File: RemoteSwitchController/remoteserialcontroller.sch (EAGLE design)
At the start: 37 parts, among them J1 ZX62R-AB-5P, J2 D-SUB9, Q2 MMSS8050-L, Q3 MMSS8050-L, SW1 SKRPACE010, SW2 SKRPACE010, U1 ADM3202ARUZ, U2 ESP-WROOM-32, U21 FT232RL

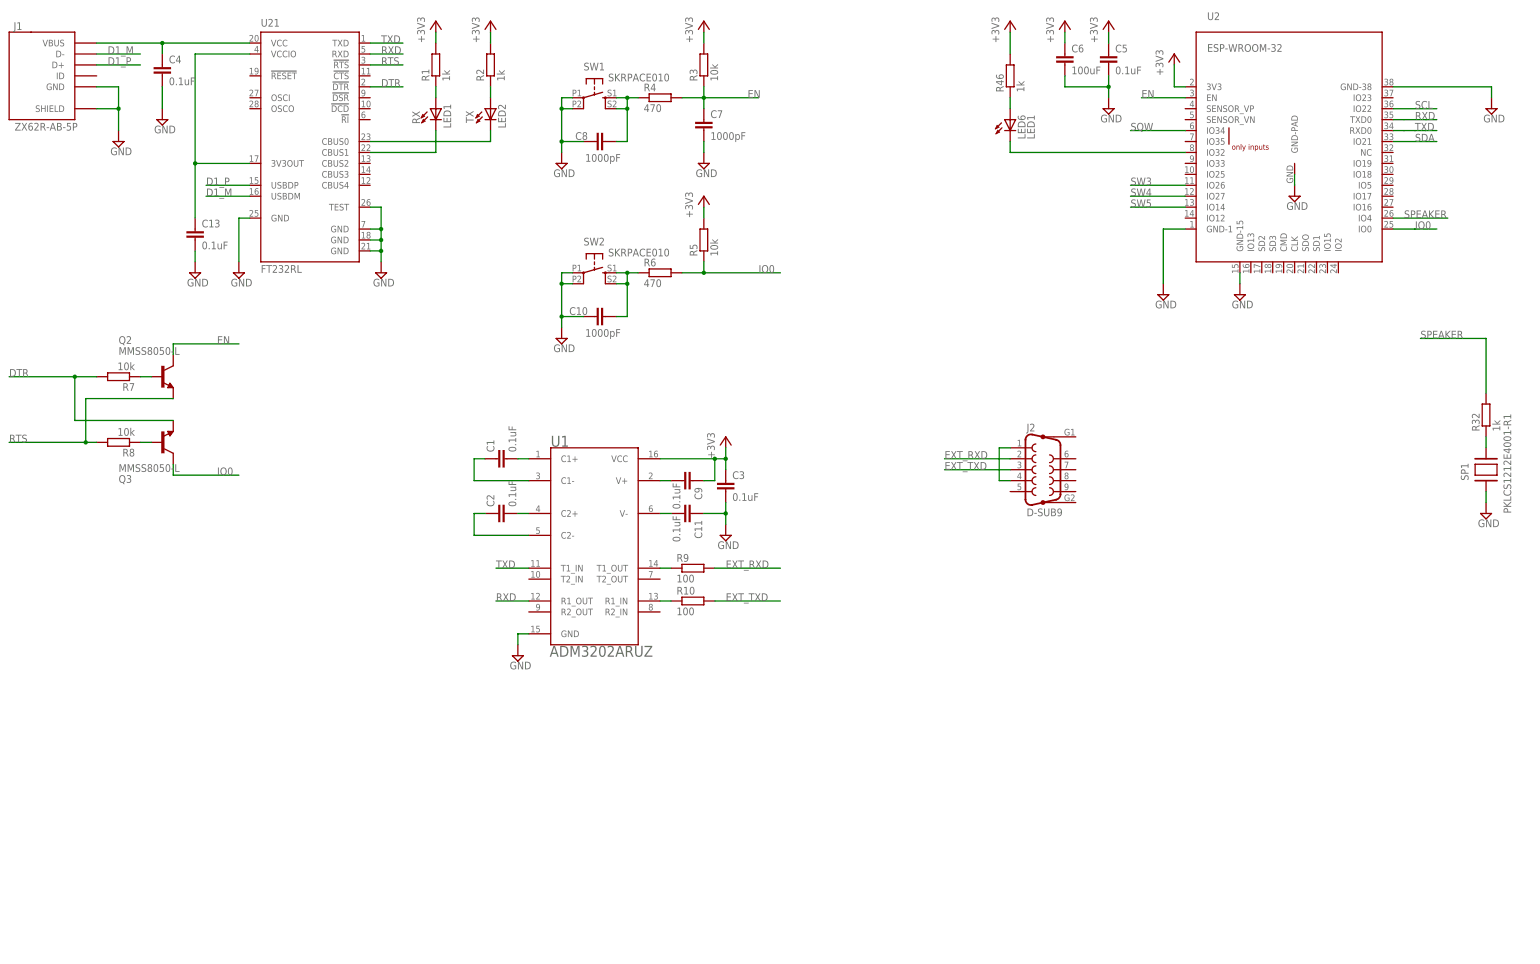
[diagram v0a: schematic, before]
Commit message: [add] temporrary
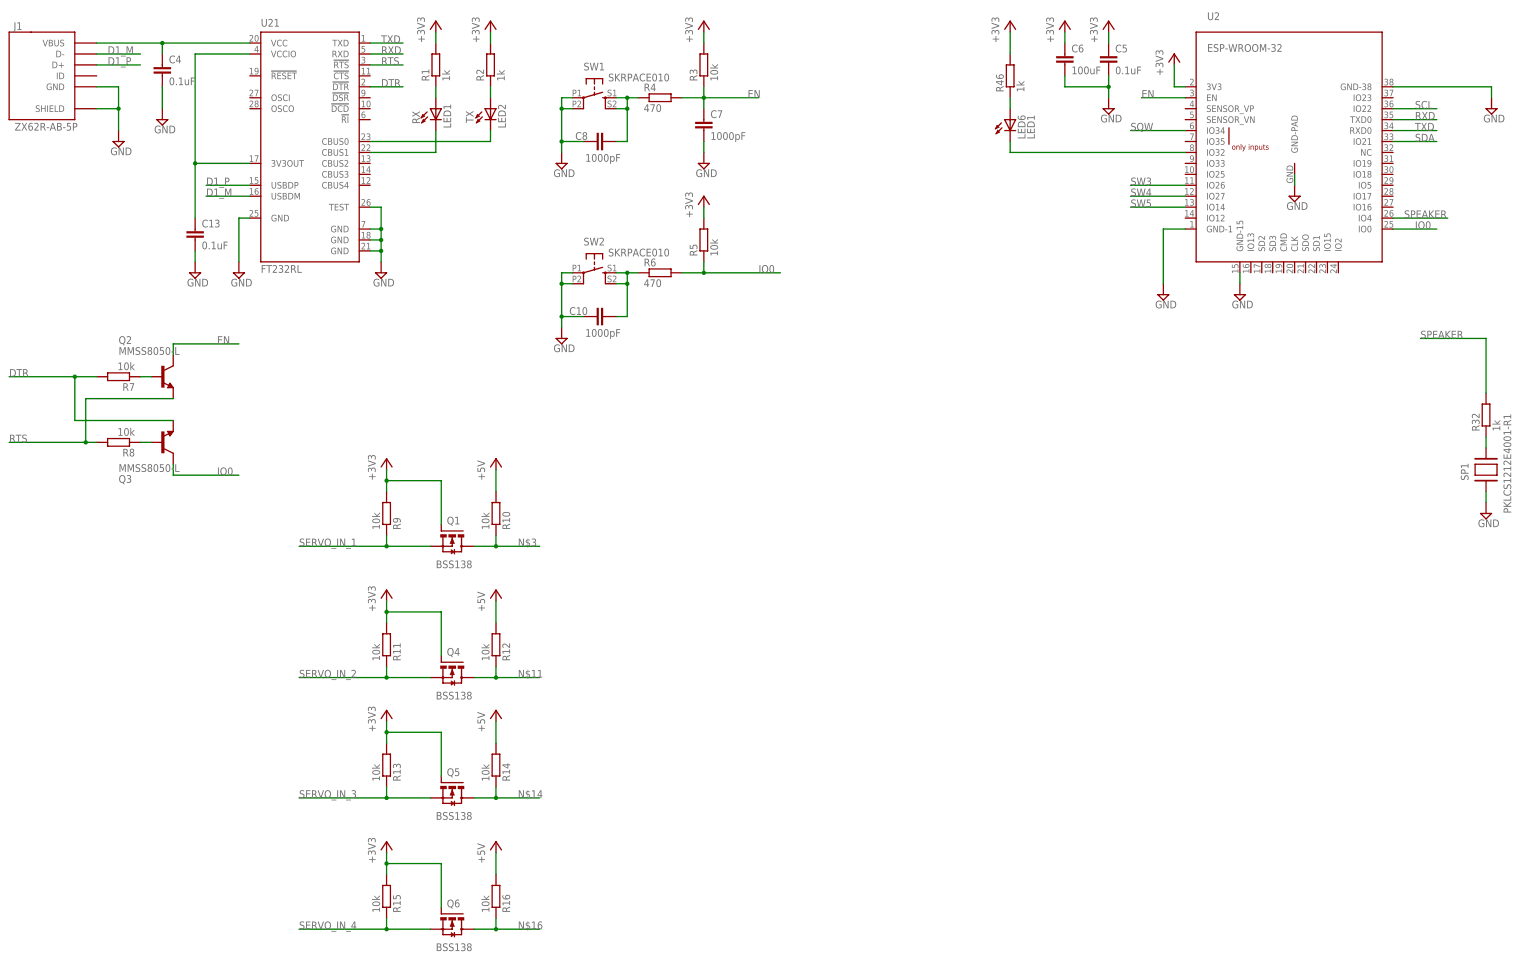
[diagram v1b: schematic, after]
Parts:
- removed C1, C11, C2, C3, C9: 0.1uF, taki-library:C-EUC0603
- removed J2: D-SUB9, taki-library:D-SUB9
- removed U1: ADM3202ARUZ, taki-library:ADM3202ARUZ
- added Q1, Q4, Q5, Q6: BSS138, taki-library:BSS138
- added R11, R12, R13, R14, R15, R16: 10k, taki-library:R-EU_R0603
- R10, R9: value 100 -> 10k
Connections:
- removed net EXT_RXD: J2.2, R9.2
- removed net EXT_TXD: J2.3, R10.2
- removed net N$1: J2.1, J2.4
- removed net N$13: C1.1, U1.C1-
- removed net N$15: C2.1, U1.C2-
- removed net N$17: C11.2, U1.V-
- removed net N$2: R9.1, U1.T1_OUT
- new net +5V: R10.2, R12.2, R14.2, R16.2
- new net SERVO_IN_1: Q1.S, R9.1
- new net SERVO_IN_2: Q4.S, R11.1
- new net SERVO_IN_3: Q5.S, R13.1
- new net SERVO_IN_4: Q6.S, R15.1
- net +3V3: now also Q1.G, Q4.G, Q5.G, Q6.G, R11.2, R13.2, R15.2, R9.2; no longer C3.1, C9.1, U1.VCC
- net GND: no longer C11.1, C3.2, U1.GND
- net N$11: now also Q4.D, R12.1; no longer C1.2, U1.C1+
- net N$14: now also Q5.D, R14.1; no longer C2.2, U1.C2+
- net N$16: now also Q6.D, R16.1; no longer C9.2, U1.V+
- net N$3: now also Q1.D; no longer U1.R1_IN
- net RXD: no longer U1.R1_OUT
- net TXD: no longer U1.T1_IN
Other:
- moved on the sheet: R10, R9

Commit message: [add]add all
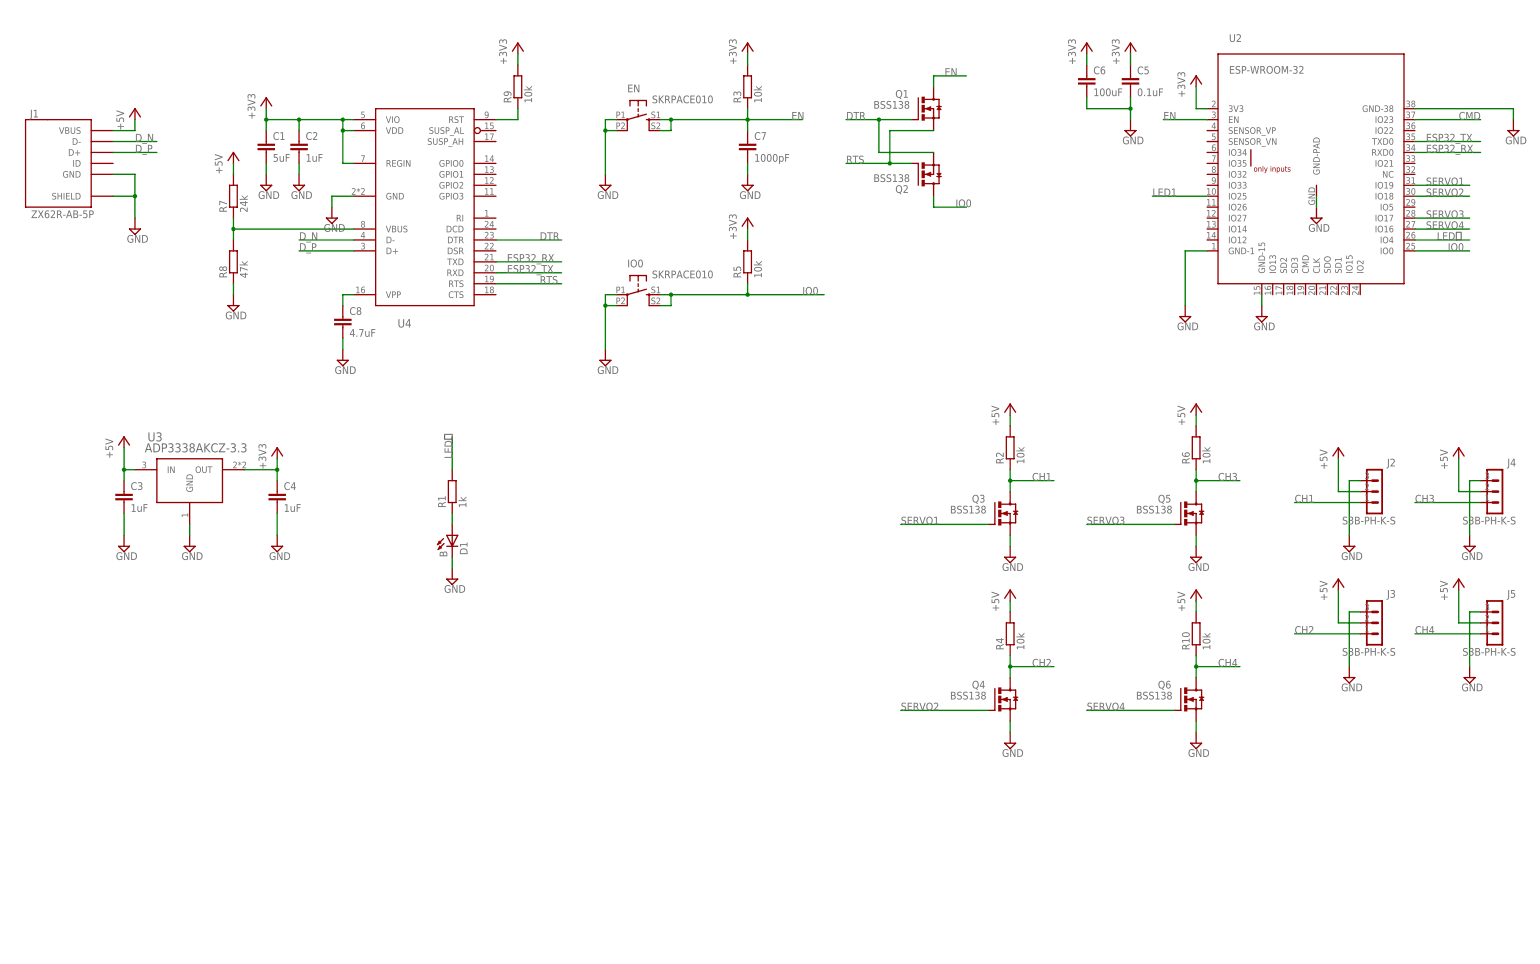
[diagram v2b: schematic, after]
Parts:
- removed C10: 1000pF, taki-library:C-EUC0603
- removed C13: 0.1uF, taki-library:C-EUC0603
- removed LED1: RX, taki-library:LEDCHIPLED_0603
- removed LED2: TX, taki-library:LEDCHIPLED_0603
- removed LED6: LED1, taki-library:LEDCHIPLED_0603
- removed R11, R12, R13, R14, R15, R16: 10k, taki-library:R-EU_R0603
- removed R32, R46: 1k, taki-library:R-EU_R0603
- removed SP1: PKLCS1212E4001-R1, taki-library:PKLCS1212E4001-R1
- removed SW1, SW2: SKRPACE010, taki-library:SKRPACE010
- removed U21: FT232RL, taki-library:FT232RL
- added C1: 5uF, taki-library:C-EUC0603
- added C2, C3: 1uF, taki-library:C-EUC0603
- added D1: B, taki-library:LEDCHIPLED_0603
- added EN, IO0: SKRPACE010, taki-library:SKRPACE010
- added J2, J3, J4, J5: S3B-PH-K-S, taki-library:S3B-PH-K-S
- added U3: ADP3338AKCZ-3.3, taki-library:ADP3338AKCZ-3.3
- added U4: CP2104, taki-library:CP2104
- C4: value 0.1uF -> 1uF
- C8: value 1000pF -> 4.7uF
- Q2, Q3: value MMSS8050-L -> BSS138; device taki-library:MMSS8050-L -> taki-library:BSS138
- R2: value 1k -> 10k
- R4, R6: value 470 -> 10k
- R7: value 10k -> 24k
- R8: value 10k -> 47k
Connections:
- removed net D1_M: J1.D-, U21.USBDM
- removed net D1_P: J1.D+, U21.USBDP
- removed net N$10: Q3.B, R8.1
- removed net N$11: Q4.D, R12.1
- removed net N$12: C10.2, R6.1, SW2.S, SW2.S1
- removed net N$14: Q5.D, R14.1
- removed net N$16: Q6.D, R16.1
- removed net N$3: Q1.D, R10.1
- removed net N$37: R32.1, SP1.1
- removed net N$4: LED1.C, U21.CBUS1
- removed net N$5: LED2.C, U21.CBUS0
- removed net N$50: LED6.C, U2.IO32
- removed net N$6: C8.2, R4.1, SW1.S, SW1.S1
- removed net N$84: C13.1, U21.3V3OUT, U21.VCCIO
- removed net N$85: C4.1, J1.VBUS, U21.VCC
- removed net RXD: U2.TXD0, U21.RXD
- removed net SCL: U2.IO22
- removed net SDA: U2.IO21
- removed net SERVO_IN_1: Q1.S, R9.1
- removed net SERVO_IN_2: Q4.S, R11.1
- removed net SERVO_IN_3: Q5.S, R13.1
- removed net SERVO_IN_4: Q6.S, R15.1
- removed net SPEAKER: R32.2, U2.IO4
- removed net SQW: U2.IO34
- removed net SW3: U2.IO26
- removed net SW4: U2.IO27
- removed net SW5: U2.IO14
- removed net TXD: U2.RXD0, U21.TXD
- new net CH1: J2.1, Q3.D, R2.1
- new net CH2: J3.1, Q4.D, R4.1
- new net CH3: J4.1, Q5.D, R6.1
- new net CH4: J5.1, Q6.D, R10.1
- new net CMD: U2.IO23
- new net D_N: J1.D-, U4.D-
- new net D_P: J1.D+, U4.D+
- new net ESP32_RX: U2.RXD0, U4.TXD
- new net ESP32_TX: U2.TXD0, U4.RXD
- new net LED1: U2.IO25
- new net LED１: R1.2, U2.IO4
- new net SERVO1: Q3.G, U2.IO19
- new net SERVO2: Q4.G, U2.IO18
- new net SERVO3: Q5.G, U2.IO17
- new net SERVO4: Q6.G, U2.IO16
- net +3V3: now also C1.1, C2.1, C4.1, U3.OUT, U4.REGIN, U4.VDD, U4.VIO; no longer Q1.G, Q4.G, Q5.G, Q6.G, R1.2, R11.2, R13.2, R15.2, R2.2, R46.2
- net +5V: now also C3.1, J1.VBUS, J2.2, J3.2, J4.2, J5.2, R2.2, R4.2, R6.2, R7.2, U3.IN; no longer R12.2, R14.2, R16.2
- net DTR: now also Q1.G, Q2.S, U4.DTR; no longer Q3.E, R7.2, U21.!DTR
- net EN: now also EN.S, EN.S1, Q1.D; no longer Q2.C, R4.2
- net GND: now also C1.2, C2.2, C3.2, C8.2, D1.C, EN.P, EN.P1, IO0.P, IO0.P1, J2.3, J3.3, J4.3, J5.3, Q3.S, Q4.S, Q5.S, Q6.S, R8.1, U3.GND, U4.GND; no longer C10.1, C13.2, C8.1, SP1.P$2, SW1.P, SW1.P1, SW2.P, SW2.P1, U21.GND, U21.GND@1, U21.GND@2, U21.GND@A, U21.TEST
- net IO0: now also IO0.S, IO0.S1, Q2.D; no longer Q3.C, R6.2
- net N$7: now also R9.1, U4.RST; no longer LED1.A, R1.1
- net N$8: now also R7.1, R8.2, U4.VBUS; no longer LED2.A, R2.1
- net N$9: now also C8.1, U4.VPP; no longer Q2.B, R7.1
- net N$94: now also D1.A, R1.1; no longer LED6.A, R46.1
- net RTS: now also Q1.S, Q2.G, U4.RTS; no longer Q2.E, R8.2, U21.!RTS
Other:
- moved on the sheet: C4, C5, C6, C7, C8, J1, Q1, Q4, Q5, Q6, R1, R10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
